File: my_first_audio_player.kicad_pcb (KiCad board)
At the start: 2 copper layers, 62.5 x 77.7 mm, 67 parts, among them J1 B2B-PH-SM4-TB(LF)(SN), J2 USB3090-XX-X_REVE, J3 SJ-3523-SMT-TR, J4 Conn_01x05_Male, J5 Conn_01x06_Male, J6 B6B-ZR(LF)(SN), J7 MEM2067-02-180-00-A_REVB, Q1 SI2333CDS-T1-GE3, U1 ADP150TUJZ3.3-EPR2, U2 MCP73826_4.1VCHCT_ND, U3 PCM1793ADB, U4 ESP32-WROOM-32, U5 OPA2134, U6 LTC1983ES6-5TRMPBF, U7 ADP150TUJZ3.3-EPR2

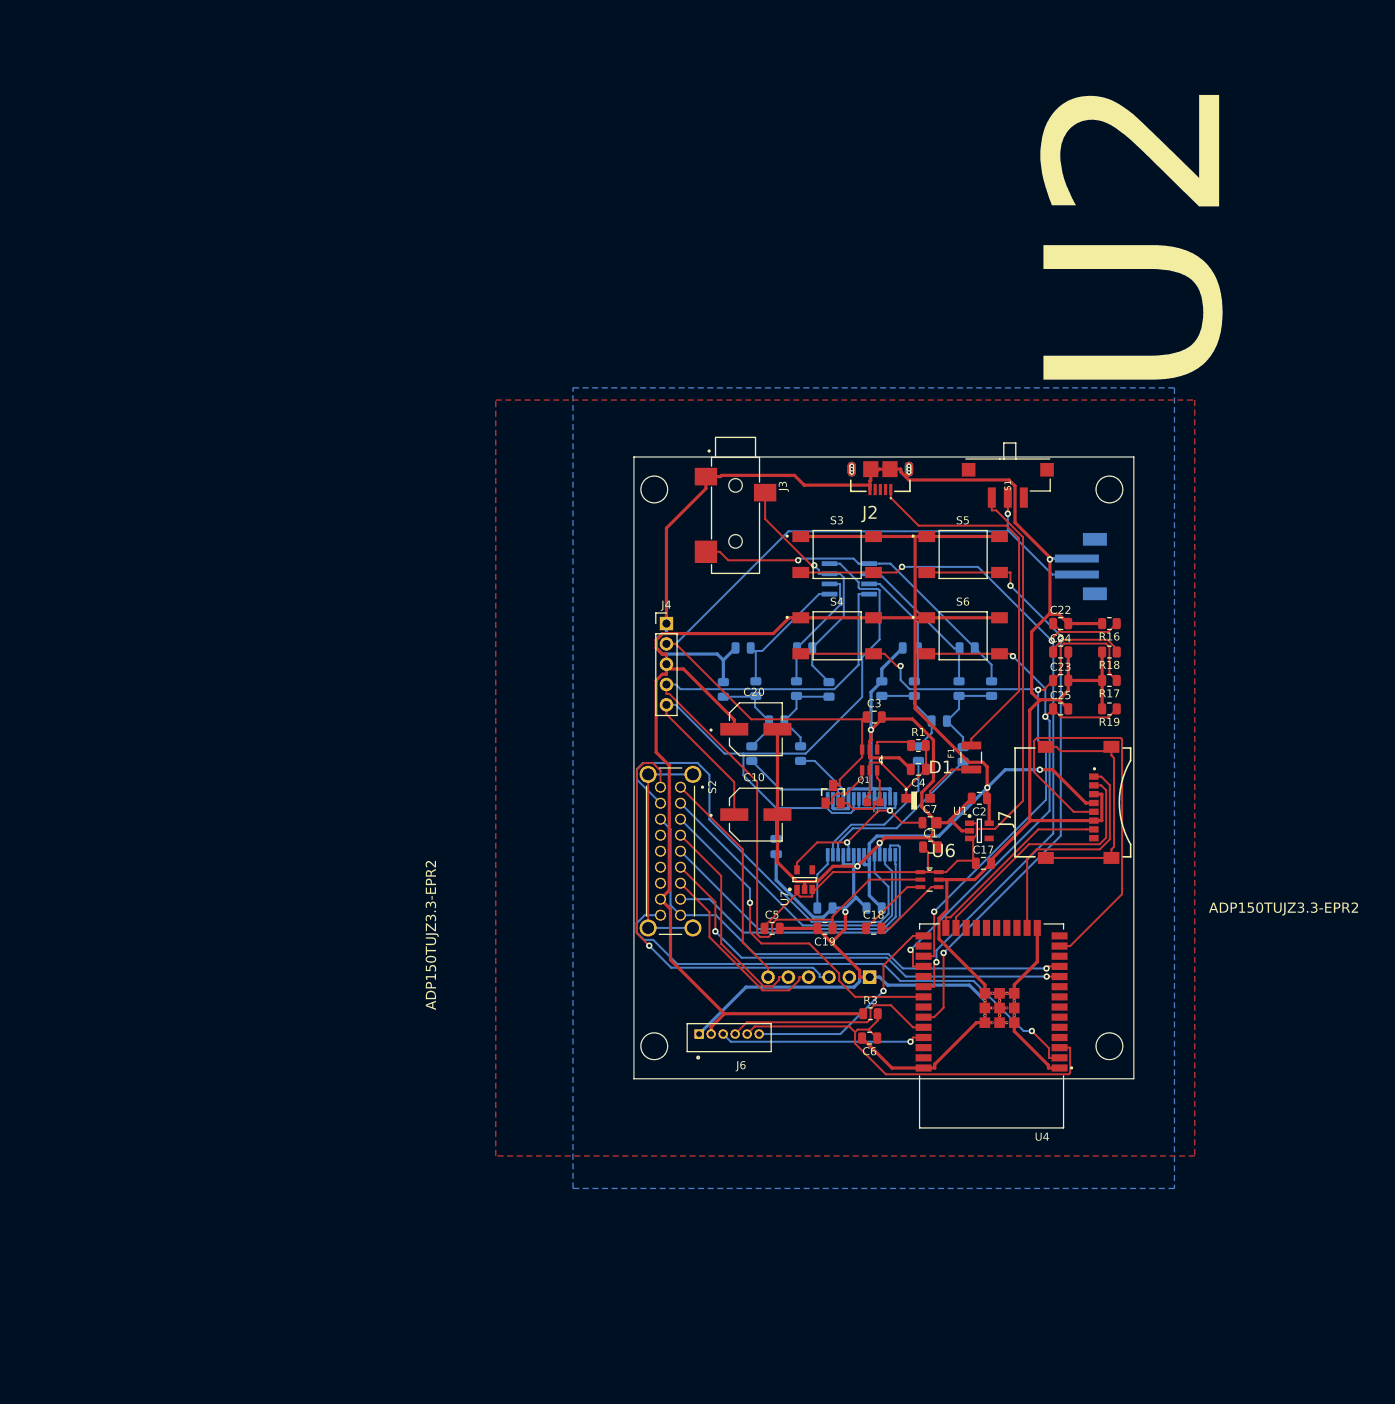
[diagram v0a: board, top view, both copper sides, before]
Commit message: [Minor] 久しぶりの謎コミットなのでバグあるかもしれないです (develop)
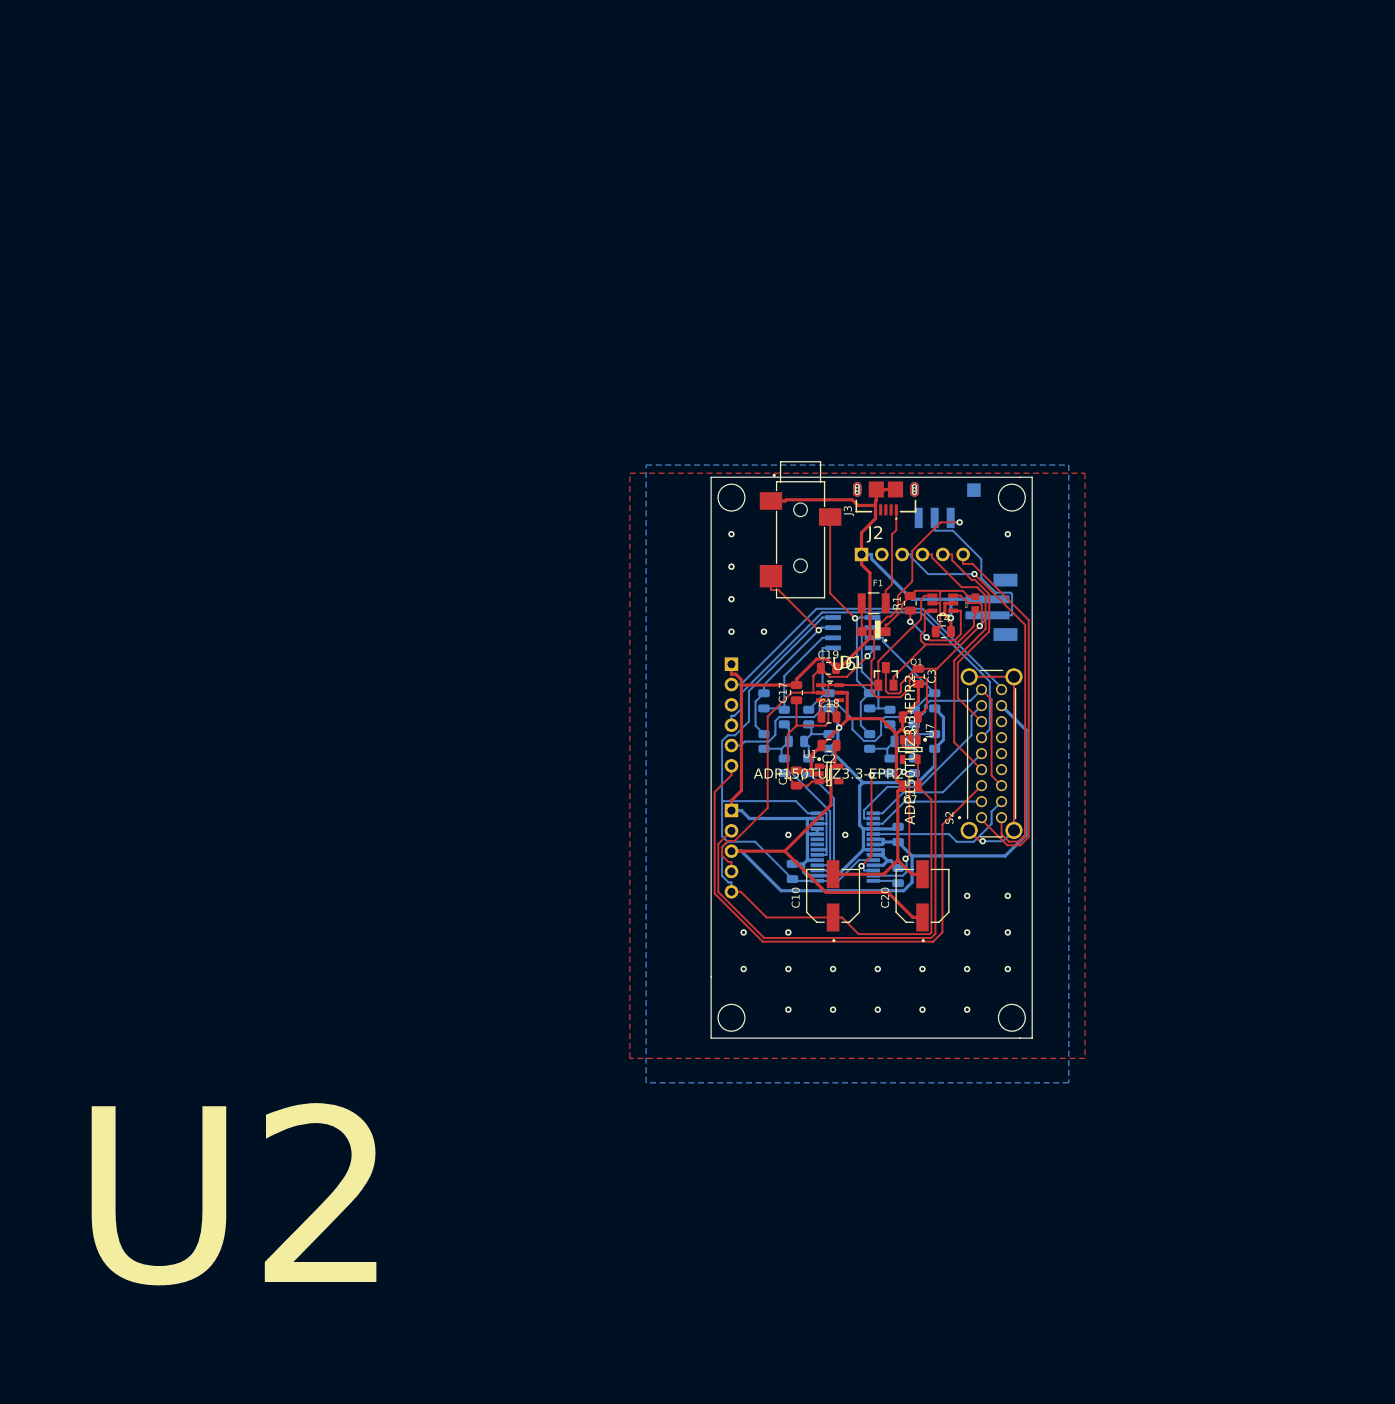
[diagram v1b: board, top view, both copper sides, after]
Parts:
- removed C22, C23, C24, C25, C6: 0.1u, Capacitor_SMD:C_0805_2012Metric
- removed J7: MEM2067-02-180-00-A_REVB, MEM2067-02-180-00-A_REVB:GCT_MEM2067-02-180-00-A_REVB
- removed R16, R17, R18, R19: 10k, Resistor_SMD:R_0805_2012Metric
- removed R3: 47k, Resistor_SMD:R_0805_2012Metric
- removed S3, S4, S5, S6: 2-1437565-8, 2-1437565-8:SW_2-1437565-8
- removed U4: ESP32-WROOM-32, ESP32-WROOM-32:MODULE_ESP32-WROOM-32
- J4, S1: moved to B.Cu
- J6: value B6B-ZR(LF)(SN) -> Conn_01x06_Male; footprint B6B-ZR_LF_SN:JST_B6B-ZR(LF)(SN) -> Connector_PinSocket_2.54mm:PinSocket_1x06_P2.54mm_Vertical; moved to B.Cu
- moved J5 52.8 mm to (129.5, 65.5), turned to 270 degrees
- moved J6 46.2 mm to (113.3, 79.2)
- moved S2 41.9 mm to (145.8, 90.4), turned to 90 degrees
- moved C19 32.5 mm to (125.4, 79.8), turned to 0 degrees
- moved C17 31.6 mm to (121.4, 82.8), turned to 90 degrees
- moved C5 31.6 mm to (135.6, 85.9), turned to 180 degrees
- moved C20 29.5 mm to (137.2, 108.2), turned to 90 degrees
- moved R2 27.9 mm to (143.8, 71.6), turned to 90 degrees
- moved C18 27.0 mm to (125.5, 85.9)
- moved U6 26.5 mm to (125.6, 82.8)
- moved J4 24.7 mm to (113.3, 97.5), turned to 180 degrees
- moved F1 22.8 mm to (131.1, 71.6), turned to 0 degrees
- moved U2 21.6 mm to (139.7, 71.6), turned to 180 degrees
- moved D1 21.6 mm to (131.1, 75.2), turned to 180 degrees
- moved U7 20.9 mm to (135.6, 89.9), turned to 270 degrees
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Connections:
- J3 pad 2: /R-CHAN -> /L-CHAN
- J3 pad 3: /L-CHAN -> /R-CHAN
- J5 pad 4: /BCK_U_I2S -> /LRCK_U_I2S
- J5 pad 5: /LRCK_U_I2S -> /BCK_U_I2S
- J6 pad 2: /+3V3 -> /CPU_+3V3
- J6 pad 3: /TXD0 -> /SCK_C_I2S
- J6 pad 4: /RXD0 -> /LRCK_C_I2S
- J6 pad 5: /CPU_EN -> /BCK_C_I2S
- J6 pad 6: /BOOT -> /DATA_C_I2S
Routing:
- net GND: track 465.7 -> 246.3 mm, vias 5 -> 12
- net /+3V3: track 239.6 -> 112.5 mm, vias 2 -> 0
- net /SW3: track 96.8 -> 0.00 mm, vias 3 -> 0
- net /SW1: track 91.4 -> 0.00 mm, vias 3 -> 0
- net /SW4: track 86.5 -> 0.00 mm, vias 3 -> 0
- net /SW2: track 70.4 -> 0.00 mm, vias 3 -> 0
- net /SD_SCK: track 54.5 -> 0.00 mm
- net /-VCC: track 97.3 -> 42.9 mm, vias 0 -> 1
- net /CPU_EN: track 54.4 -> 0.00 mm
- net /SCK: track 57.3 -> 19.4 mm
- net Net-(F1-Pad2): track 47.5 -> 12.2 mm
- net /SD_MOSI: track 31.9 -> 0.00 mm
- net Net-(J7-Pad10): track 30.8 -> 0.00 mm
- net /SD_CS: track 29.2 -> 0.00 mm
- net /BOOT: track 27.5 -> 0.00 mm, vias 1 -> 0
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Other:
- board size 62.5 x 77.7 mm -> 40.1 x 70.1 mm
